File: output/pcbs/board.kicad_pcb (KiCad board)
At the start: 2 copper layers, 94 x 86 mm, 38 parts

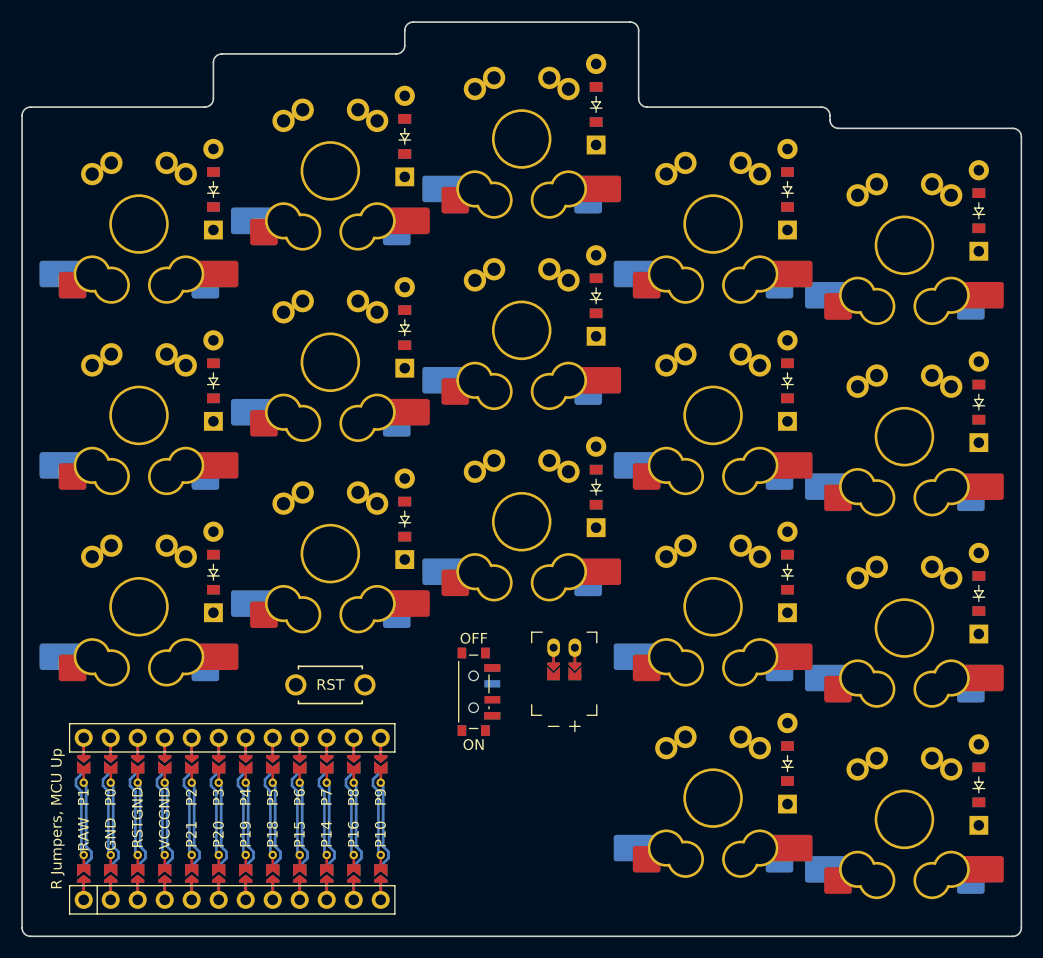
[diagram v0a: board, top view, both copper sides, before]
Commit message: final
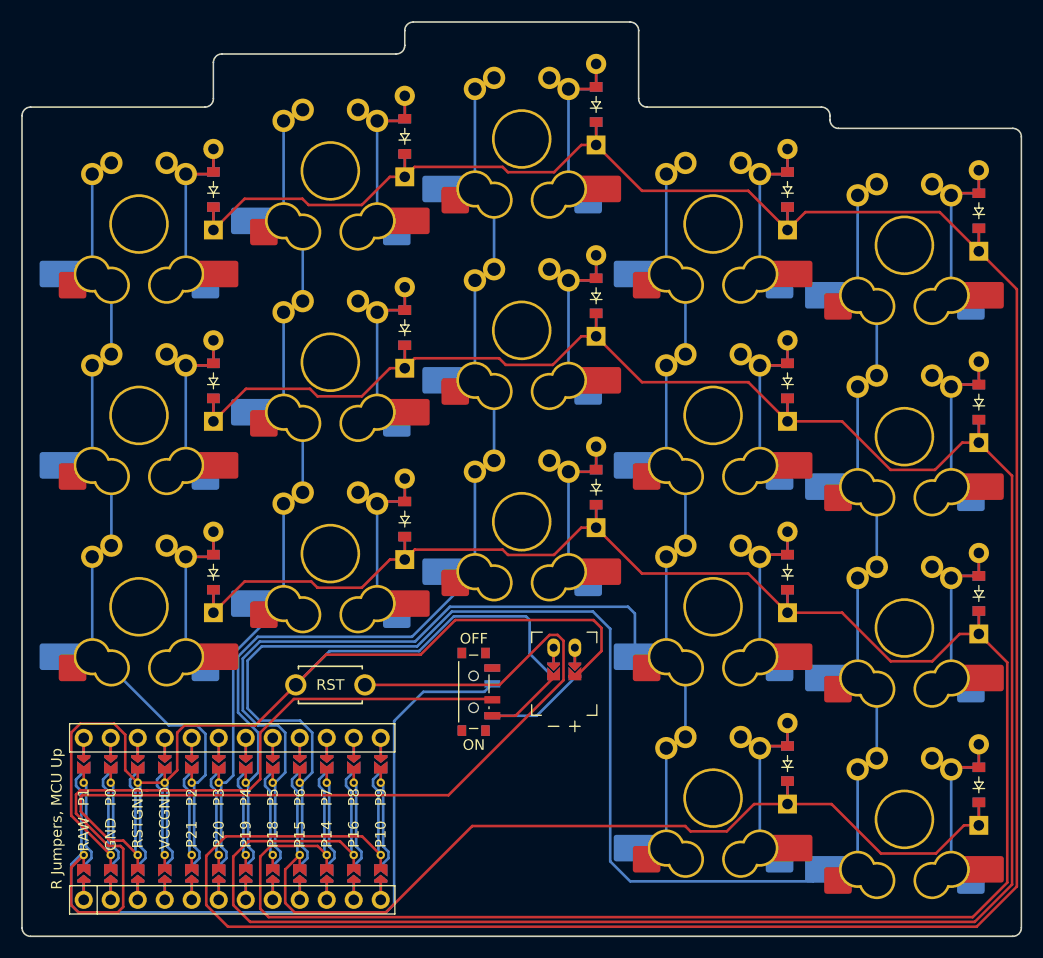
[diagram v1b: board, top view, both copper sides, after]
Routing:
- net (no net): track 337.7 -> 0.00 mm
- net P10: track 0.00 -> 275.6 mm
- net P16: track 0.00 -> 249.4 mm
- net P14: track 0.00 -> 222.3 mm
- net P6: track 0.00 -> 163.9 mm
- net RAW: track 0.00 -> 143.2 mm
- net GND: track 0.00 -> 142.6 mm
- net P5: track 0.00 -> 125.2 mm
- net P15: track 0.00 -> 96.8 mm
- net RST: track 0.00 -> 93.1 mm
- net P4: track 0.00 -> 91.2 mm
- net P3: track 0.00 -> 70.8 mm
- net P2: track 0.00 -> 67.9 mm
- net index_bottom: track 0.00 -> 20.9 mm
- net middle_bottom: track 0.00 -> 19.6 mm
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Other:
- net class Default removed

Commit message: Revert "final"
This reverts commit 3cc0ae3dbf9a7bfc7c0c773b724c9739fb3c472e.
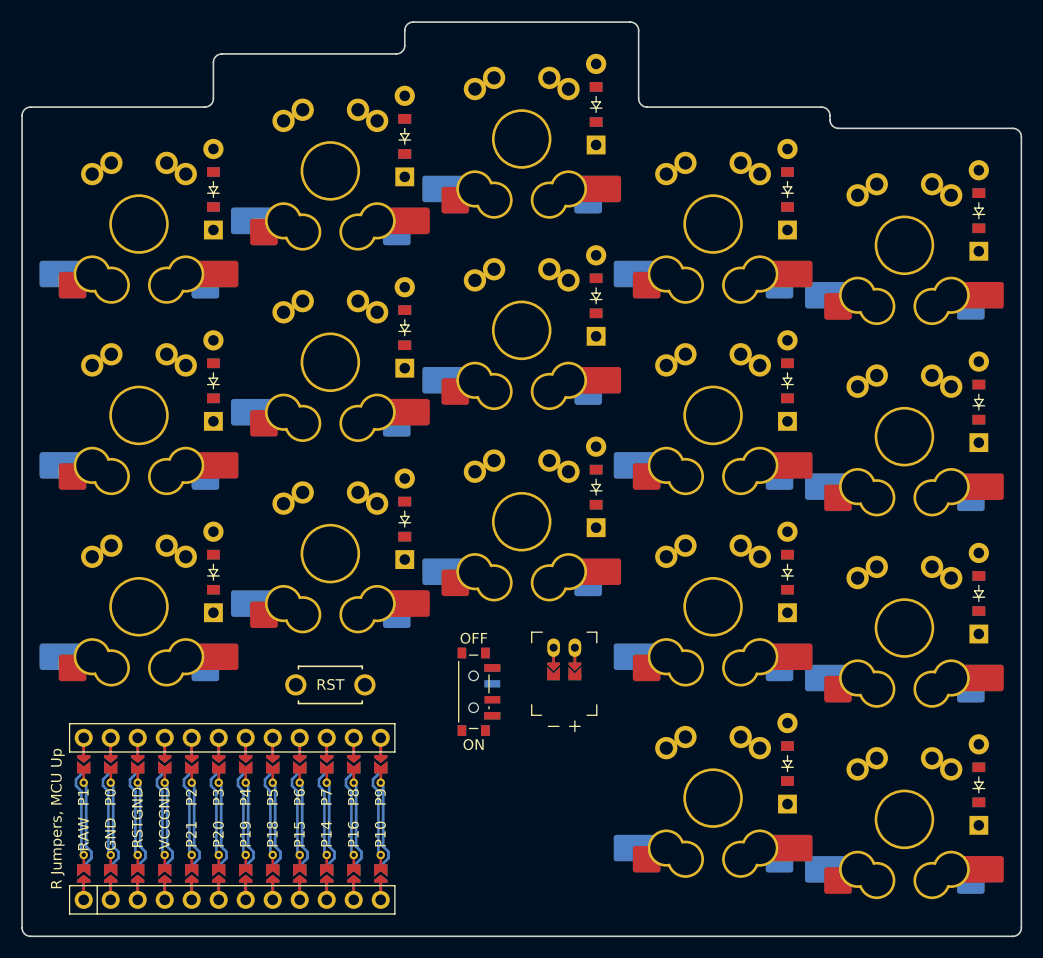
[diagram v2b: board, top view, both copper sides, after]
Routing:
- net (no net): track 0.00 -> 337.7 mm
- net P10: track 275.6 -> 0.00 mm
- net P16: track 249.4 -> 0.00 mm
- net P14: track 222.3 -> 0.00 mm
- net P6: track 163.9 -> 0.00 mm
- net RAW: track 143.2 -> 0.00 mm
- net GND: track 142.6 -> 0.00 mm
- net P5: track 125.2 -> 0.00 mm
- net P15: track 96.8 -> 0.00 mm
- net RST: track 93.1 -> 0.00 mm
- net P4: track 91.2 -> 0.00 mm
- net P3: track 70.8 -> 0.00 mm
- net P2: track 67.9 -> 0.00 mm
- net index_bottom: track 20.9 -> 0.00 mm
- net middle_bottom: track 19.6 -> 0.00 mm
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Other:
- net class Default added: clearance 0.2, trace_width 0.25, via_dia 0.8, via_drill 0.4
